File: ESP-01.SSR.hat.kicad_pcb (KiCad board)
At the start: 2 copper layers, 45.1 x 35.6 mm, 12 parts, among them J1 Screw_Terminal_01x02, J2 Screw_Terminal_01x02, J3 Screw_Terminal_01x02, K1 G3MB-202P, K2 G3MB-202P, Q1 BC547, Q2 BC547, U1 ESP-01v090, U2 AMS1117-3.3

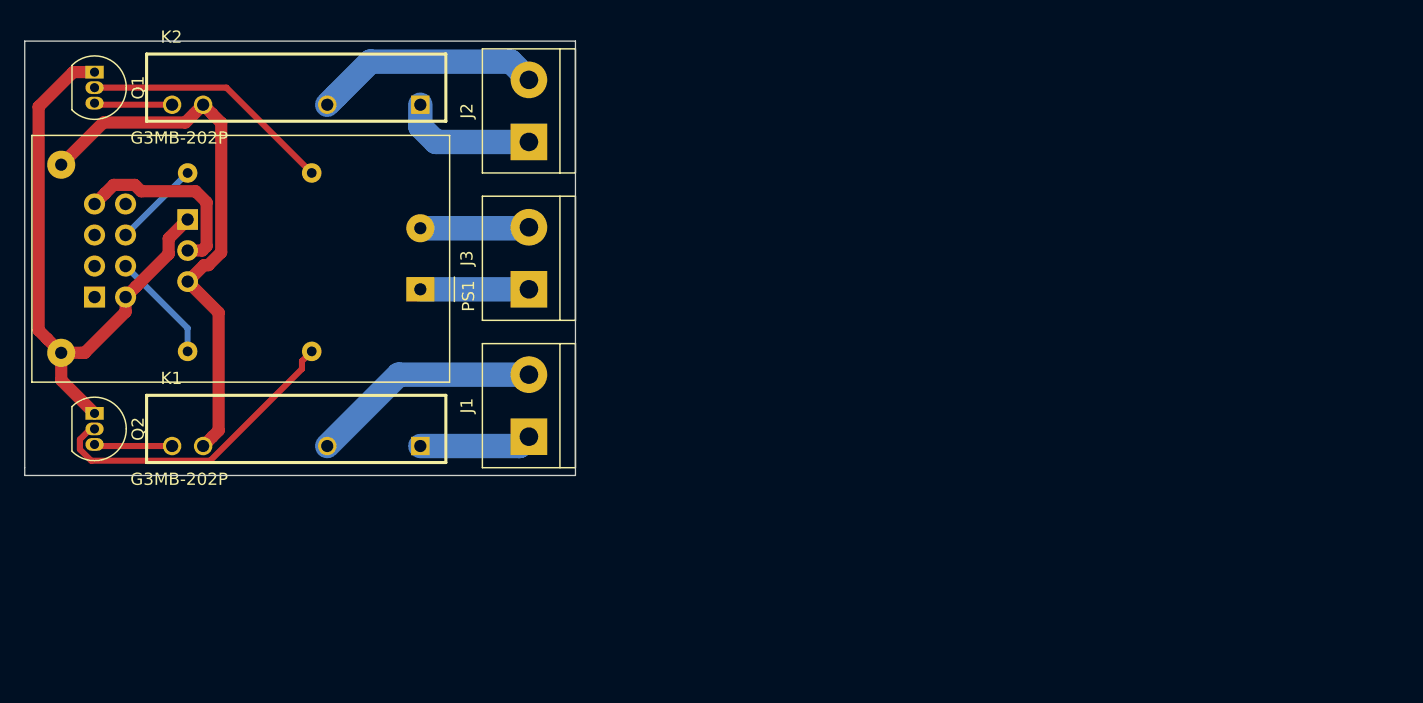
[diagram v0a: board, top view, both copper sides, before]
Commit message: board redesign
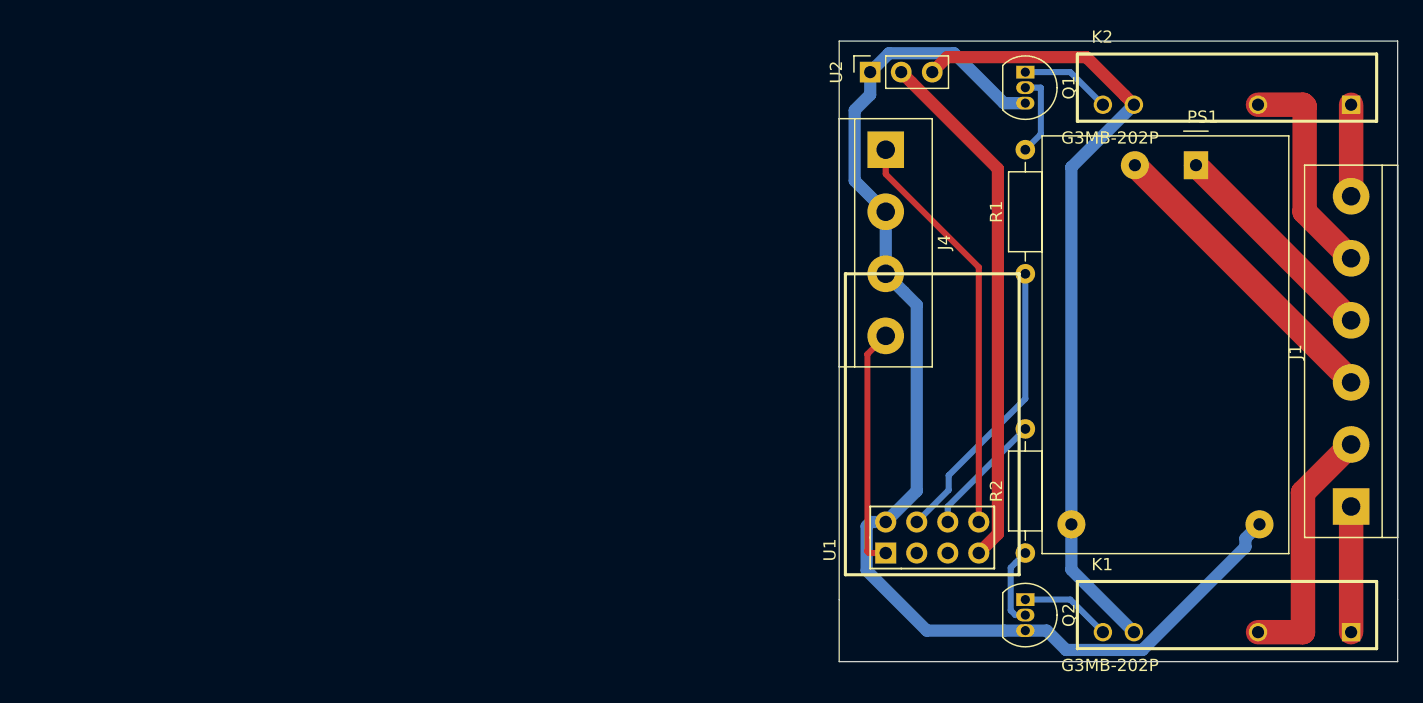
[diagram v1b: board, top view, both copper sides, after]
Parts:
- removed J2, J3: Screw_Terminal_01x02, TerminalBlock:TerminalBlock_bornier-2_P5.08mm
- added J4: Screw_Terminal_01x04, TerminalBlock:TerminalBlock_bornier-4_P5.08mm, F.Cu at (171.4, 33.0)
- J1: value Screw_Terminal_01x02 -> Screw_Terminal_01x06; footprint TerminalBlock:TerminalBlock_bornier-2_P5.08mm -> TerminalBlock:TerminalBlock_bornier-6_P5.08mm
- R1: value R -> 4k7; moved to F.Cu
- R2: value R -> 20k; moved to F.Cu
- U1: moved to F.Cu
- U2: footprint Connector_PinSocket_2.54mm:PinSocket_1x03_P2.54mm_Horizontal -> Connector_PinSocket_2.54mm:PinSocket_1x03_P2.54mm_Vertical; moved to F.Cu
- moved K1 77.7 mm to (199.4, 71.1)
- moved Q2 77.7 mm to (182.9, 69.8)
- moved K2 76.2 mm to (199.4, 27.9)
- moved Q1 76.2 mm to (182.9, 26.7)
- moved R1 69.1 mm to (182.9, 43.2), turned to 90 degrees
- moved U1 68.1 mm to (171.4, 66.0), turned to 90 degrees
- moved J1 67.6 mm to (209.6, 62.2)
- moved PS1 64.3 mm to (196.8, 34.3), turned to 270 degrees
- moved R2 60.7 mm to (182.9, 66.0), turned to 90 degrees
- moved U2 57.2 mm to (170.2, 26.7), turned to 90 degrees
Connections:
- K2 pad 1: Net-(J2-Pad1) -> Net-(J1-Pad6)
- K2 pad 2: Net-(J2-Pad2) -> Net-(J1-Pad5)
- PS1 pad 1: Net-(J3-Pad1) -> Net-(J1-Pad4)
- PS1 pad 2: Net-(J3-Pad2) -> Net-(J1-Pad3)
- Q1 pad 1: GND -> Net-(K2-Pad4)
- Q1 pad 3: Net-(K2-Pad4) -> GND
- Q2 pad 1: GND -> Net-(K1-Pad4)
- Q2 pad 3: Net-(K1-Pad4) -> GND
- U1 pad 3: Net-(U1-Pad3) -> (no net)
- U1 pad 4: Net-(R2-Pad2) -> Net-(R1-Pad1)
- U1 pad 5: Net-(U1-Pad5) -> (no net)
- U1 pad 6: Net-(R1-Pad1) -> Net-(R2-Pad2)
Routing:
- net GND: track 49.3 -> 100.4 mm
- net Net-(J4-Pad1): track 0.00 -> 33.6 mm
- net +3.3V: track 15.7 -> 43.3 mm
- net Net-(J1-Pad3): track 0.00 -> 25.1 mm
- net +5V: track 45.1 -> 66.1 mm
- net Net-(J4-Pad4): track 0.00 -> 19.8 mm
- net Net-(Q2-Pad2): track 25.8 -> 6.55 mm
- net Net-(J2-Pad2): track 18.6 -> 0.00 mm
- net Net-(J1-Pad4): track 0.00 -> 18.0 mm
- net Net-(J1-Pad5): track 0.00 -> 17.9 mm
- net Net-(R1-Pad1): track 7.18 -> 24.0 mm
- net Net-(Q1-Pad2): track 20.7 -> 6.86 mm
- net Net-(J2-Pad1): track 11.2 -> 0.00 mm
- net Net-(J3-Pad2): track 8.92 -> 0.00 mm
- net Net-(J3-Pad1): track 8.89 -> 0.00 mm
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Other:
- board size 45.1 x 35.6 mm -> 45.7 x 50.8 mm
